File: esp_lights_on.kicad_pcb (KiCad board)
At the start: 2 copper layers, 50 x 60 mm, 19 parts, among them J2 Conn_01x06_Pin, J3 VIN, J4 Screw_Terminal_01x03, K1 RELAY, K2 RELAY, Q1 SS8050, Q2 SS8050, U1 ESP32-WROOM-32, U2 TLV1117-33

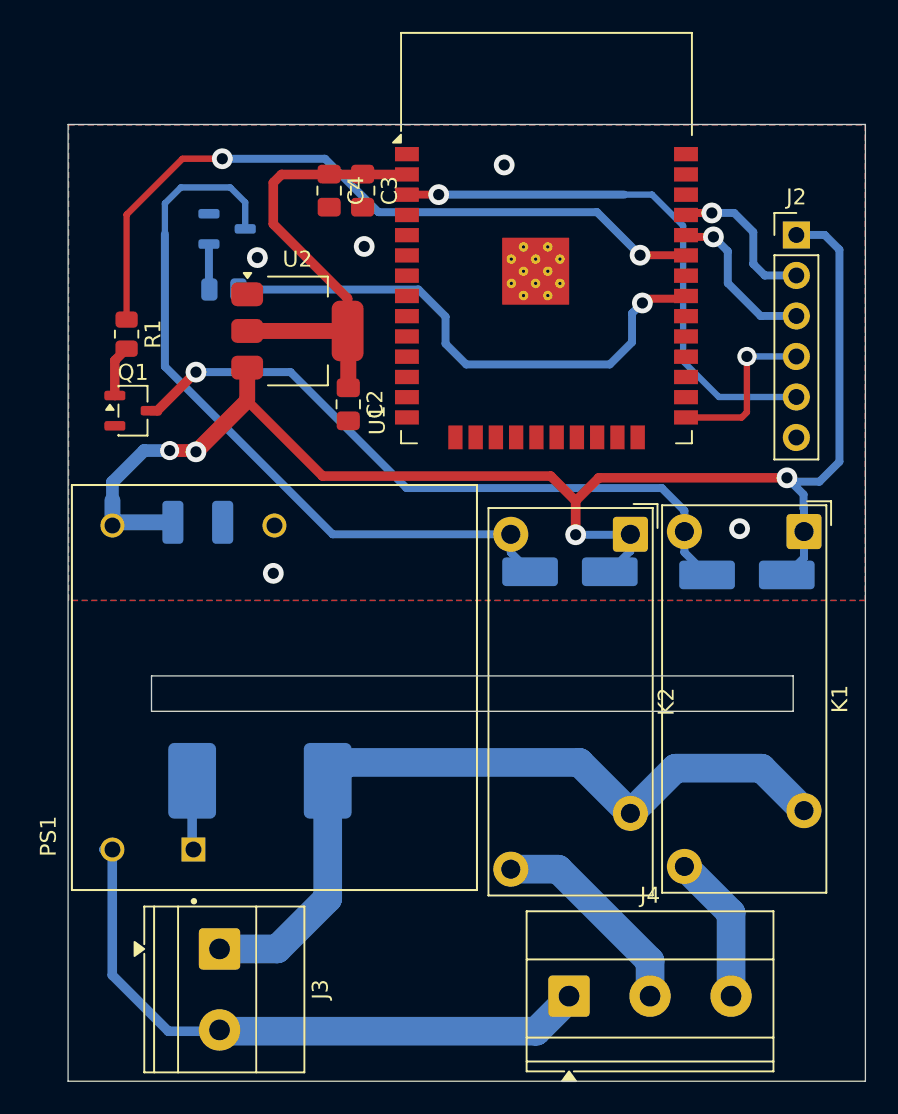
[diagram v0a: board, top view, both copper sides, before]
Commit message: fixes
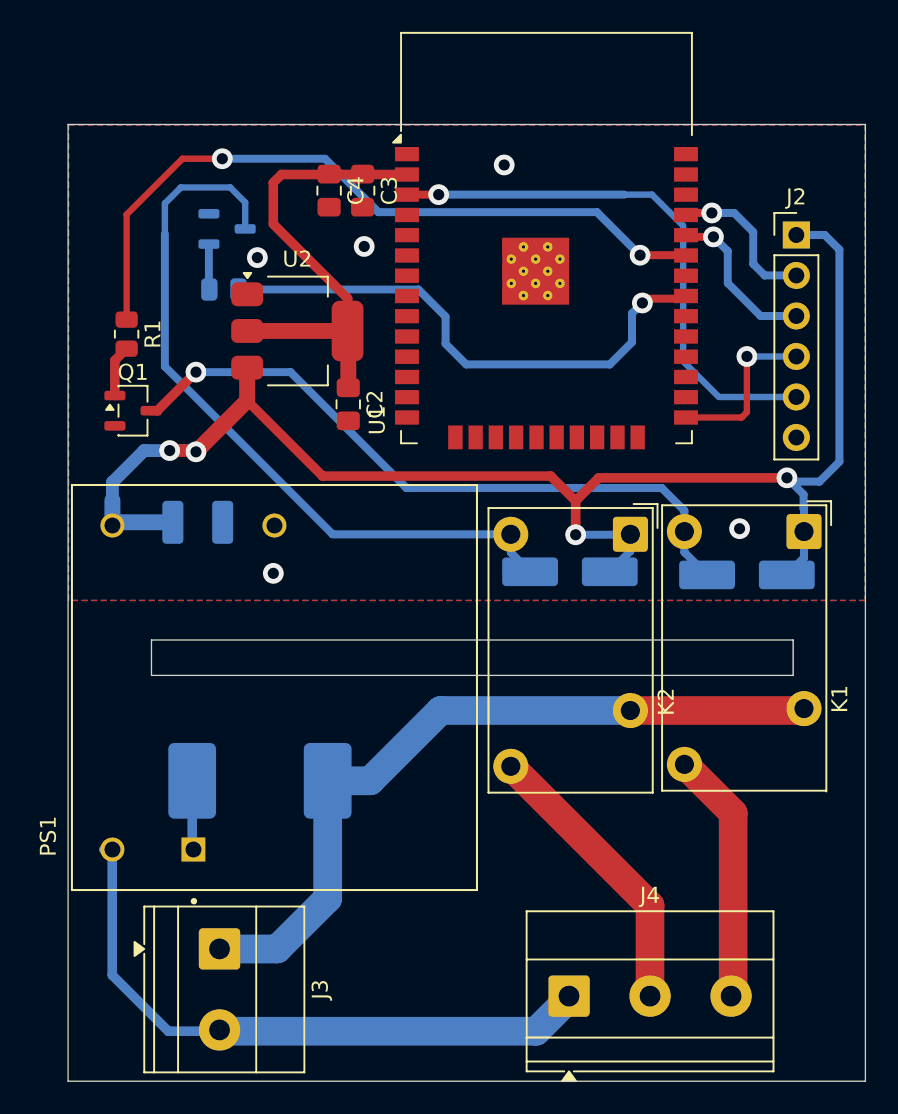
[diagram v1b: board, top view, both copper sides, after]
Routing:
- net circuit1: track 9.34 -> 15.9 mm
- net circuit2: track 13.3 -> 18.0 mm
- net VIN_220V: track 49.4 -> 47.2 mm
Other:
- outline, holes or cut-outs redrawn

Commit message: other fixes
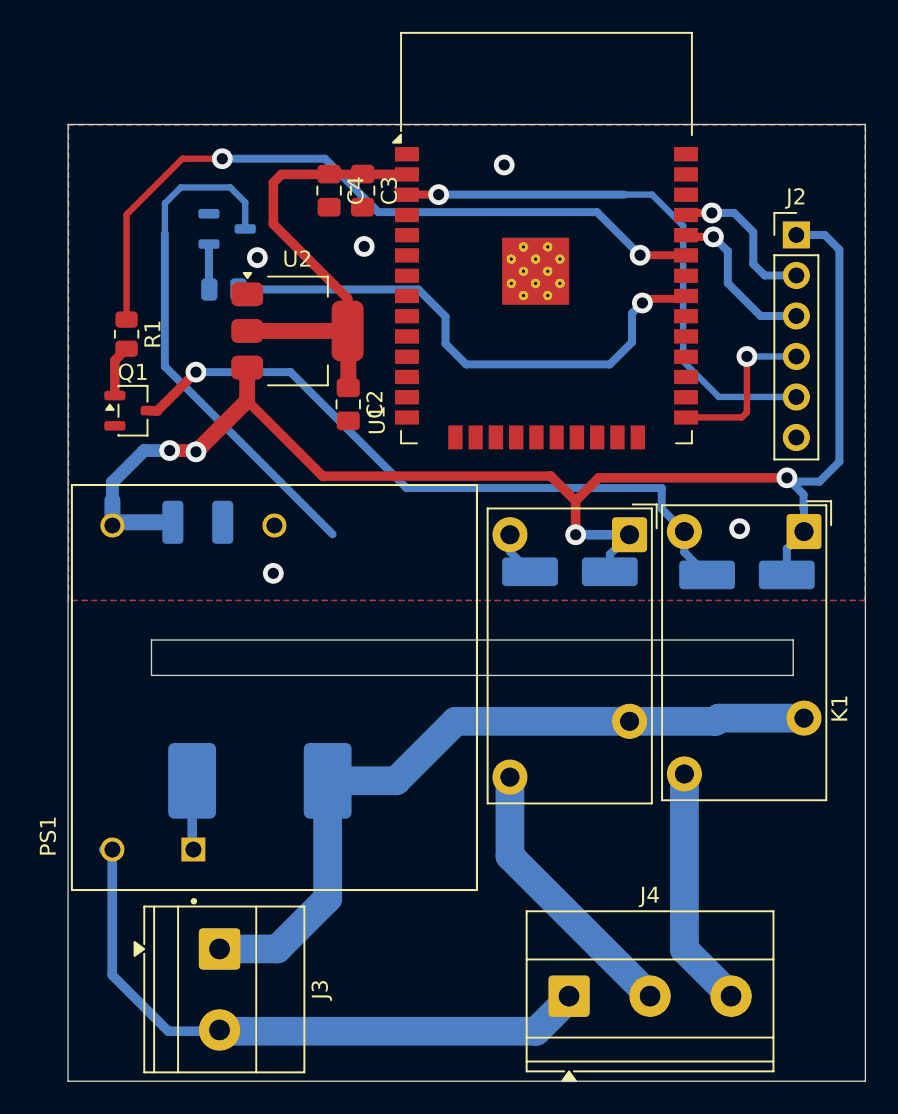
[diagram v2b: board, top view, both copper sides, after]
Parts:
- moved K2 2.01 mm to (226.2, 55.4)
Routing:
- net COLECTOR2: track 46.4 -> 35.3 mm
- net circuit2: track 18.0 -> 17.4 mm
- net circuit1: track 15.9 -> 15.3 mm
